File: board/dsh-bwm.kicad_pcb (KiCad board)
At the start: 2 copper layers, 121.3 x 78.7 mm, 37 parts, among them IC1 TPS5450DDA, IC2 MAX485CSA+T, J1 MPM-15-24, J2 Power, J3 Connections, J4 LED, J5 SWD6p, K1 833H-1C-C-24VDC, K2 833H-1C-C-24VDC, K3 833H-1C-C-24VDC, K4 833H-1C-C-24VDC, Q1 IRLB8721PBF, SW1 BOOTSEL, U1 RP2040_Stamp

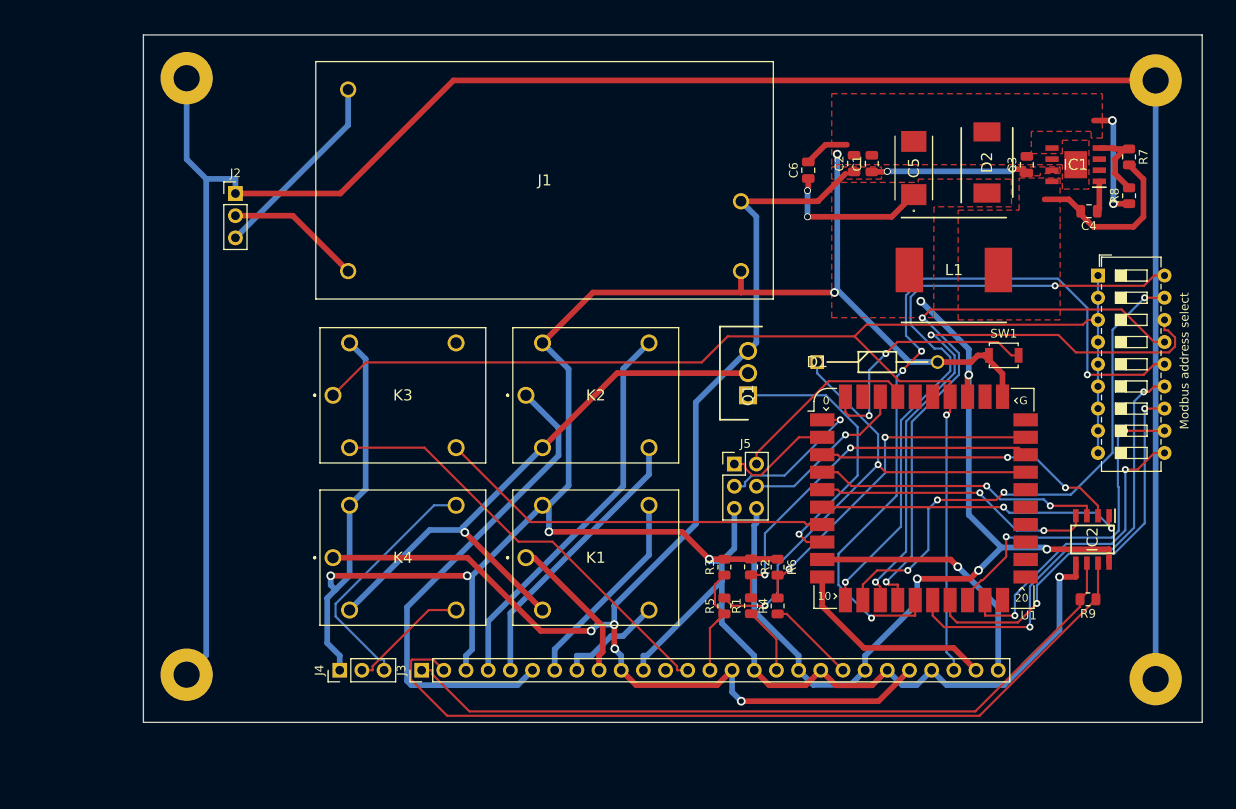
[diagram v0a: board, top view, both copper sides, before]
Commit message: TPs, vias, some comments on board, fml
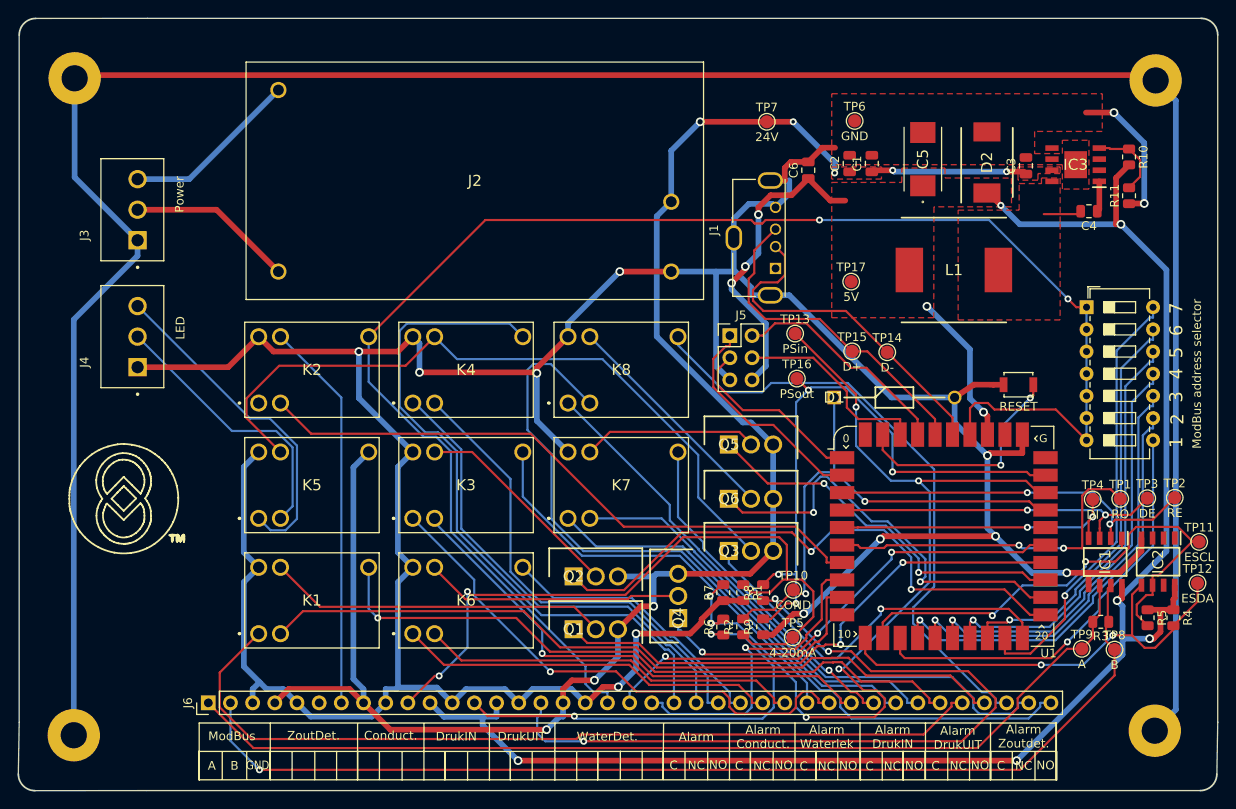
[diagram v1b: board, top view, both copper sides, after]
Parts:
- removed the J3 at (123.4, 128.0)
- removed Modbus address select: SW_DIP_x09, Button_Switch_THT:SW_DIP_SPSTx09_Slide_6.7x24.42mm_W7.62mm_P2.54mm_LowProfile
- removed the R1 at (161.2, 120.6)
- removed the R2 at (161.2, 116.2)
- added IC2: AT24C256C-SSHL-T, SamacSys_Parts:SOIC127P600X175-8N, F.Cu at (207.8, 115.6)
- added J1: USB_A, Connector_USB:USB_A_Molex_105057_Vertical, F.Cu at (164.0, 82.0)
- added J6: Connections, Connector_PinHeader_2.54mm:PinHeader_1x39_P2.54mm_Vertical, F.Cu at (99.0, 131.8)
- added K1: T81N5D312, SamacSys_Parts:T81H5D31212, F.Cu at (104.8, 123.8)
- added K6: T81N5D312, SamacSys_Parts:T81H5D31212, F.Cu at (122.4, 123.8)
- added K7: T81N5D312, SamacSys_Parts:T81H5D31212, F.Cu at (140.2, 110.6)
- added K8: T81N5D312, SamacSys_Parts:T81H5D31212, F.Cu at (140.2, 97.4)
- added Q1: IRLB8721PBF, SamacSys_Parts:TO254P483X1016X1994-3P, F.Cu at (140.8, 123.3)
- added Q2: IRLB8721PBF, SamacSys_Parts:TO254P483X1016X1994-3P, F.Cu at (140.8, 117.3)
- added Q4: IRLB8721PBF, SamacSys_Parts:TO254P483X1016X1994-3P, F.Cu at (152.8, 122.0)
- added Q5: IRLB8721PBF, SamacSys_Parts:TO254P483X1016X1994-3P, F.Cu at (158.6, 102.2)
- added Q6: IRLB8721PBF, SamacSys_Parts:TO254P483X1016X1994-3P, F.Cu at (158.6, 108.4)
- added R5: 10k, Resistor_SMD:R_0805_2012Metric, F.Cu at (206.6, 122.0)
- added R7: 2k, Resistor_SMD:R_0805_2012Metric, F.Cu at (158.0, 119.1)
- added R8: 1k, Resistor_SMD:R_0805_2012Metric, F.Cu at (162.6, 119.1)
- added R9: 2k, Resistor_SMD:R_0805_2012Metric, F.Cu at (162.6, 123.0)
- added SW2: RESET, Button_Switch_SMD:SW_SPST_B3U-1000P, F.Cu at (191.8, 95.3)
- added TP1: RO, TestPoint:TestPoint_Pad_D1.5mm, F.Cu at (203.5, 108.4)
- added TP10: COND, TestPoint:TestPoint_Pad_D1.5mm, F.Cu at (166.0, 118.8)
- added TP11: ESCL, TestPoint:TestPoint_Pad_D1.5mm, F.Cu at (212.5, 113.3)
- added TP12: ESDA, TestPoint:TestPoint_Pad_D1.5mm, F.Cu at (212.3, 118.0)
- added TP13: PSin, TestPoint:TestPoint_Pad_D1.5mm, F.Cu at (166.2, 89.5)
- added TP14: D-, TestPoint:TestPoint_Pad_D1.5mm, F.Cu at (176.8, 91.6)
- added TP15: D+, TestPoint:TestPoint_Pad_D1.5mm, F.Cu at (172.8, 91.5)
- added TP16: PSout, TestPoint:TestPoint_Pad_D1.5mm, F.Cu at (166.4, 94.6)
- added TP17: 5V, TestPoint:TestPoint_Pad_D1.5mm, F.Cu at (172.6, 83.5)
- added TP2: RE, TestPoint:TestPoint_Pad_D1.5mm, F.Cu at (209.7, 108.2)
- added TP3: DE, TestPoint:TestPoint_Pad_D1.5mm, F.Cu at (206.6, 108.3)
- added TP4: DI, TestPoint:TestPoint_Pad_D1.5mm, F.Cu at (200.3, 108.5)
- added TP5: 4-20mA, TestPoint:TestPoint_Pad_D1.5mm, F.Cu at (165.9, 124.2)
- added TP6: GND, TestPoint:TestPoint_Pad_D1.5mm, F.Cu at (173.0, 65.1)
- added TP7: 24V, TestPoint:TestPoint_Pad_D1.5mm, F.Cu at (163.0, 65.2)
- added TP8: B, TestPoint:TestPoint_Pad_D1.5mm, F.Cu at (202.8, 125.7)
- added TP9: A, TestPoint:TestPoint_Pad_D1.5mm, F.Cu at (199.1, 125.6)
- J3: renamed from J2; footprint Connector_PinHeader_2.54mm:PinHeader_1x03_P2.54mm_Vertical -> TBP03R2-350-03BE:CUI_TBP03R2-350-03BE
- J4: footprint Connector_PinHeader_2.54mm:PinHeader_1x03_P2.54mm_Vertical -> TBP03R2-350-03BE:CUI_TBP03R2-350-03BE
- K2: renamed from K3; value 833H-1C-C-24VDC -> T81N5D312; footprint SamacSys_Parts:833H1CC24VDC -> SamacSys_Parts:T81H5D31212
- K3: renamed from K1; value 833H-1C-C-24VDC -> T81N5D312; footprint SamacSys_Parts:833H1CC24VDC -> SamacSys_Parts:T81H5D31212
- K4: renamed from K2; value 833H-1C-C-24VDC -> T81N5D312; footprint SamacSys_Parts:833H1CC24VDC -> SamacSys_Parts:T81H5D31212
- K5: renamed from K4; value 833H-1C-C-24VDC -> T81N5D312; footprint SamacSys_Parts:833H1CC24VDC -> SamacSys_Parts:T81H5D31212
- R4: value 1k -> 10k
- R6: value 2k -> 1k
- SW1: value BOOTSEL -> ModBus address selector; footprint Button_Switch_SMD:SW_SPST_B3U-1000P -> Button_Switch_THT:SW_DIP_SPSTx07_Slide_6.7x19.34mm_W7.62mm_P2.54mm_LowProfile
- moved R4 45.4 mm to (209.5, 122.0), turned to -90 degrees
- moved J4 41.7 mm to (90.9, 93.3)
- moved Q3 18.0 mm to (158.6, 114.3), turned to 0 degrees
- moved J5 14.7 mm to (158.7, 89.7)
- moved H3 14.7 mm to (83.6, 135.5)
- moved K3 13.7 mm to (122.4, 110.6)
- moved K4 13.0 mm to (122.4, 97.4)
- moved H1 12.8 mm to (83.7, 60.2)
- moved J3 12.4 mm to (90.9, 78.8), turned to 90 degrees
- moved SW1 11.0 mm to (199.6, 86.4)
- moved K5 9.63 mm to (104.8, 110.6)
- moved R6 9.26 mm to (158.0, 123.1), turned to 90 degrees
- moved K2 8.56 mm to (104.8, 97.4)
- moved J2 7.99 mm to (152.0, 74.3)
- moved H2 5.91 mm to (207.4, 134.9)
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- renumbered IC2 to IC1, IC1 to IC3, J1 to J2, Q1 to Q3, R3 to R1, R7 to R10, R8 to R11, R5 to R2, R9 to R3
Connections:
- K2 pad 1: 3v3 -> unconnected-(K2-Pad1)
- K2 pad 2: ZDSENSE -> ZD
- K2 pad 3: ZD -> 3v3
- K2 pad 4: unconnected-(K3-Pad4) -> ZDSENSE
- K3 pad 1: AlarmC1 -> LekNC
- K3 pad 2: Net-(K1-Pad2) -> LekNO
- K3 pad 3: AlarmNO1 -> LekC
- K3 pad 4: AlarmNC1 -> Net-(K3-Pad4)
- K4 pad 1: AlarmC2 -> AlarmNC
- K4 pad 2: Net-(K1-Pad2) -> AlarmNO
- K4 pad 3: AlarmNO2 -> AlarmC
- K4 pad 4: AlarmNC2 -> Net-(K4-Pad4)
- K5 pad 1: 24V -> R
- K5 pad 2: Net-(K1-Pad2) -> G
- K5 pad 3: G -> 24V
- K5 pad 4: R -> Net-(K4-Pad4)
- Q3 pad 2: Net-(K1-Pad2) -> Net-(K4-Pad4)
- R10 pad 2: /Power/5Vunf -> 5V
- R4 pad 1: PressureOUT -> 5V
- R4 pad 2: PSout -> EEPROMSDA
- R6 pad 1: GND -> PressureIN
- R6 pad 2: PSout -> PSin
- SW1 pad 1: GND -> 3v3
- SW1 pad 2: Net-(SW1-Pad2) -> 3v3
- U1 pad 10: LDNC -> unconnected-(U1-Pad10)
- U1 pad 11: MBADRB1 -> EEPROMSDA
- U1 pad 12: MBADRB2 -> EEPROMSCL
- U1 pad 13: MBADRB3 -> MBADRB1
- U1 pad 14: MBADRB4 -> MBADRB2
- U1 pad 15: MBADRB5 -> MBADRB3
- U1 pad 16: MBADRB7 -> MBADRB4
- U1 pad 17: MBADRB6 -> MBADRB5
- U1 pad 18: MBADRB8 -> MBADRB6
- U1 pad 19: MBADRB9 -> MBADRB7
- U1 pad 20: unconnected-(U1-Pad20) -> ALARM
- U1 pad 21: unconnected-(U1-Pad21) -> ALARMLEK
- U1 pad 22: unconnected-(U1-Pad22) -> ALARMZOUT
- U1 pad 23: unconnected-(U1-Pad23) -> ALARMDRUKIN
- U1 pad 24: unconnected-(U1-Pad24) -> ALARMDRUKUIT
- U1 pad 25: unconnected-(U1-Pad25) -> ALARMCOND
- U1 pad 35: unconnected-(U1-Pad35) -> Net-(U1-Pad35)
- U1 pad 36: unconnected-(U1-Pad36) -> Net-(U1-Pad36)
- U1 pad 39: RESET -> Net-(U1-Pad39)
- U1 pad 40: Net-(SW1-Pad2) -> unconnected-(U1-Pad40)
- U1 pad 8: ALARM -> LDNO
- U1 pad 9: LDNO -> LDNC
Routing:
- net 5V: track 120.1 -> 236.9 mm, vias 7 -> 11
- net DrukUitNC: track 0.00 -> 98.8 mm
- net ZoutNO: track 0.00 -> 95.8 mm
- net GND: track 321.5 -> 409.6 mm, vias 9 -> 13
- net DrukUitNO: track 0.00 -> 87.2 mm
- net Net-(K4-Pad4): track 0.00 -> 81.5 mm
- net PressureOUT: track 10.2 -> 90.7 mm, vias 0 -> 3
- net AlarmC: track 0.00 -> 77.7 mm
- net DrukUitC: track 0.00 -> 75.9 mm, vias 0 -> 1
- net ZoutC: track 0.00 -> 70.5 mm
- net ZoutNC: track 0.00 -> 70.1 mm
- net Net-(K1-Pad2): track 70.0 -> 0.00 mm, vias 1 -> 0
- net 4-20mA input: track 13.7 -> 81.9 mm, vias 0 -> 2
- net ALARMLEK: track 0.00 -> 65.6 mm, vias 0 -> 2
- net PSin: track 43.2 -> 107.2 mm, vias 2 -> 6
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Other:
- board size 121.3 x 78.7 mm -> 137.4 x 88.5 mm
- board text added: "1"
- board text added: "2"
- board text added: "3"
- board text added: "4"
- board text added: "5"
- board text added: "6"
- board text added: "7"
- board text added: "A"
- board text added: "Alarm"
- board text added: "Alarm Conduct."
- board text added: "Alarm DrukIN"
- board text added: "Alarm DrukUIT"
- board text added: "Alarm Waterlek"
- board text added: "Alarm Zoutdet."
- board text added: "B"
- board text added: "C"
- board text added: "Conduct."
- board text added: "DSH Belgium Leandro Marceddu DSH WaterManager (v0.1)"
- board text added: "DrukIN"
- board text added: "DrukUIT"
- board text added: "GND"
- board text added: "ModBus"
- board text added: "NC"
- board text added: "NO"
- board text added: "WaterDet."
- board text added: "ZoutDet."
